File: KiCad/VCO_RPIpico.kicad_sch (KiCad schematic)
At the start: 30 parts, among them J1 AudioJack2, J2 Power Jack 5V, J3 Wave Out, J4 Echo Out, J5 Poti Echo Mix/Feedback, J6 Poti Echo Freq, J7 Echo Power, SW1 LFO Waveform, SW2 Shift1, SW3 Fire4, SW4 Fire3, SW5 Fire2, SW6 Fire1, SW7 Shift2, SW8 Shift3

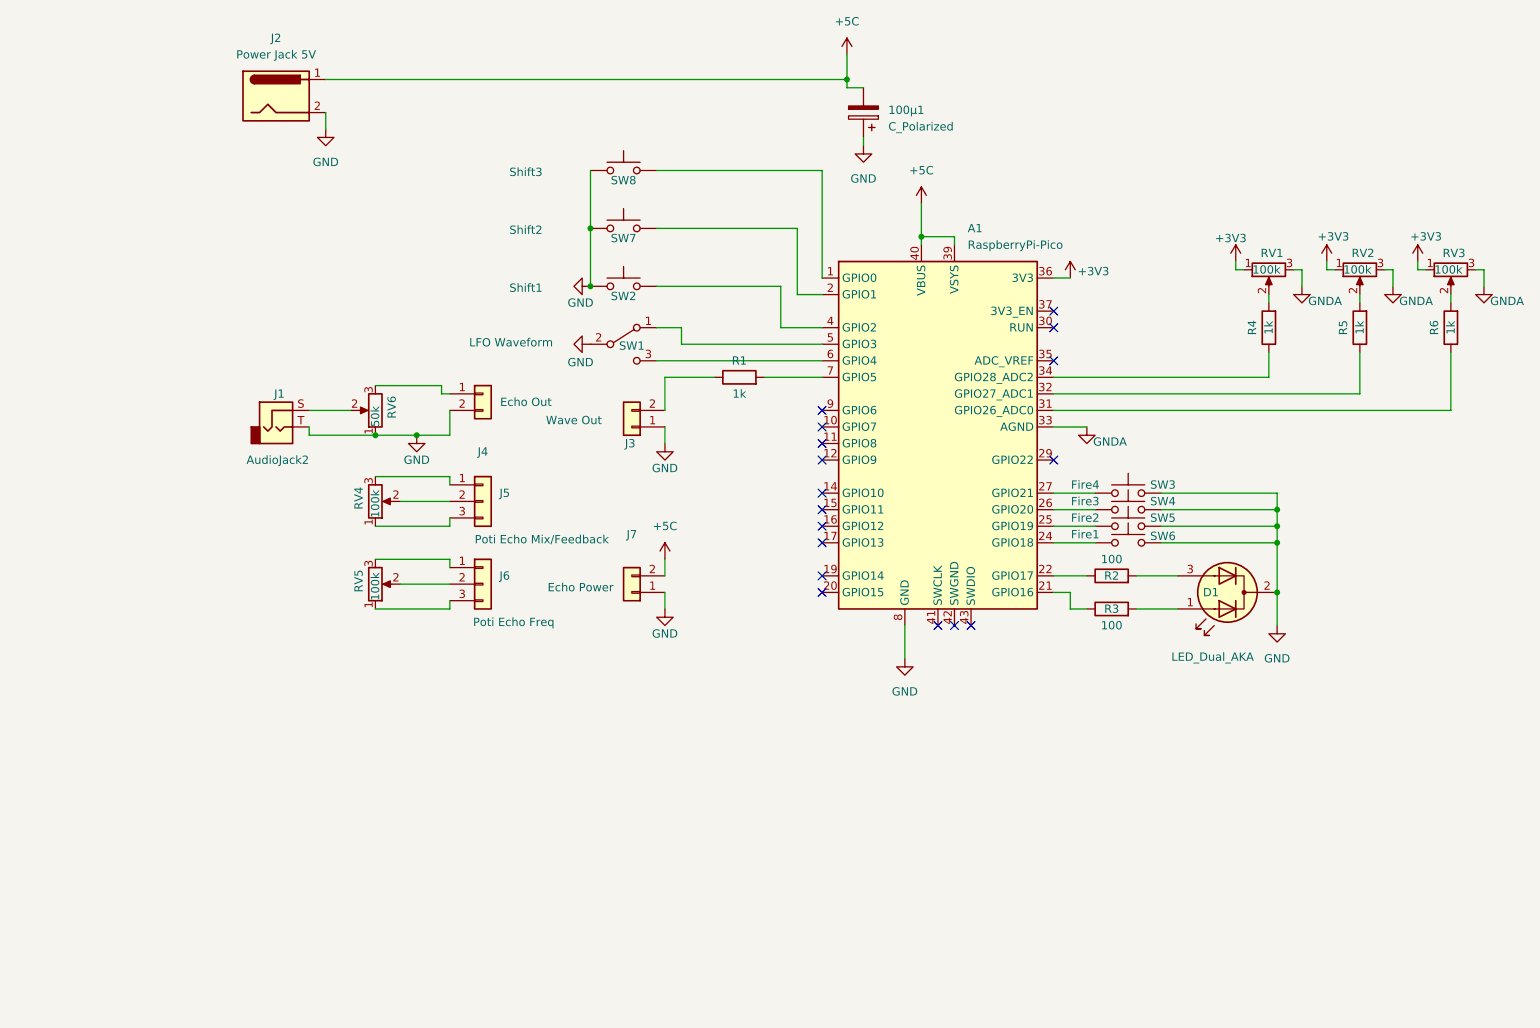
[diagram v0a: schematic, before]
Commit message: Kicad Schematic and Board
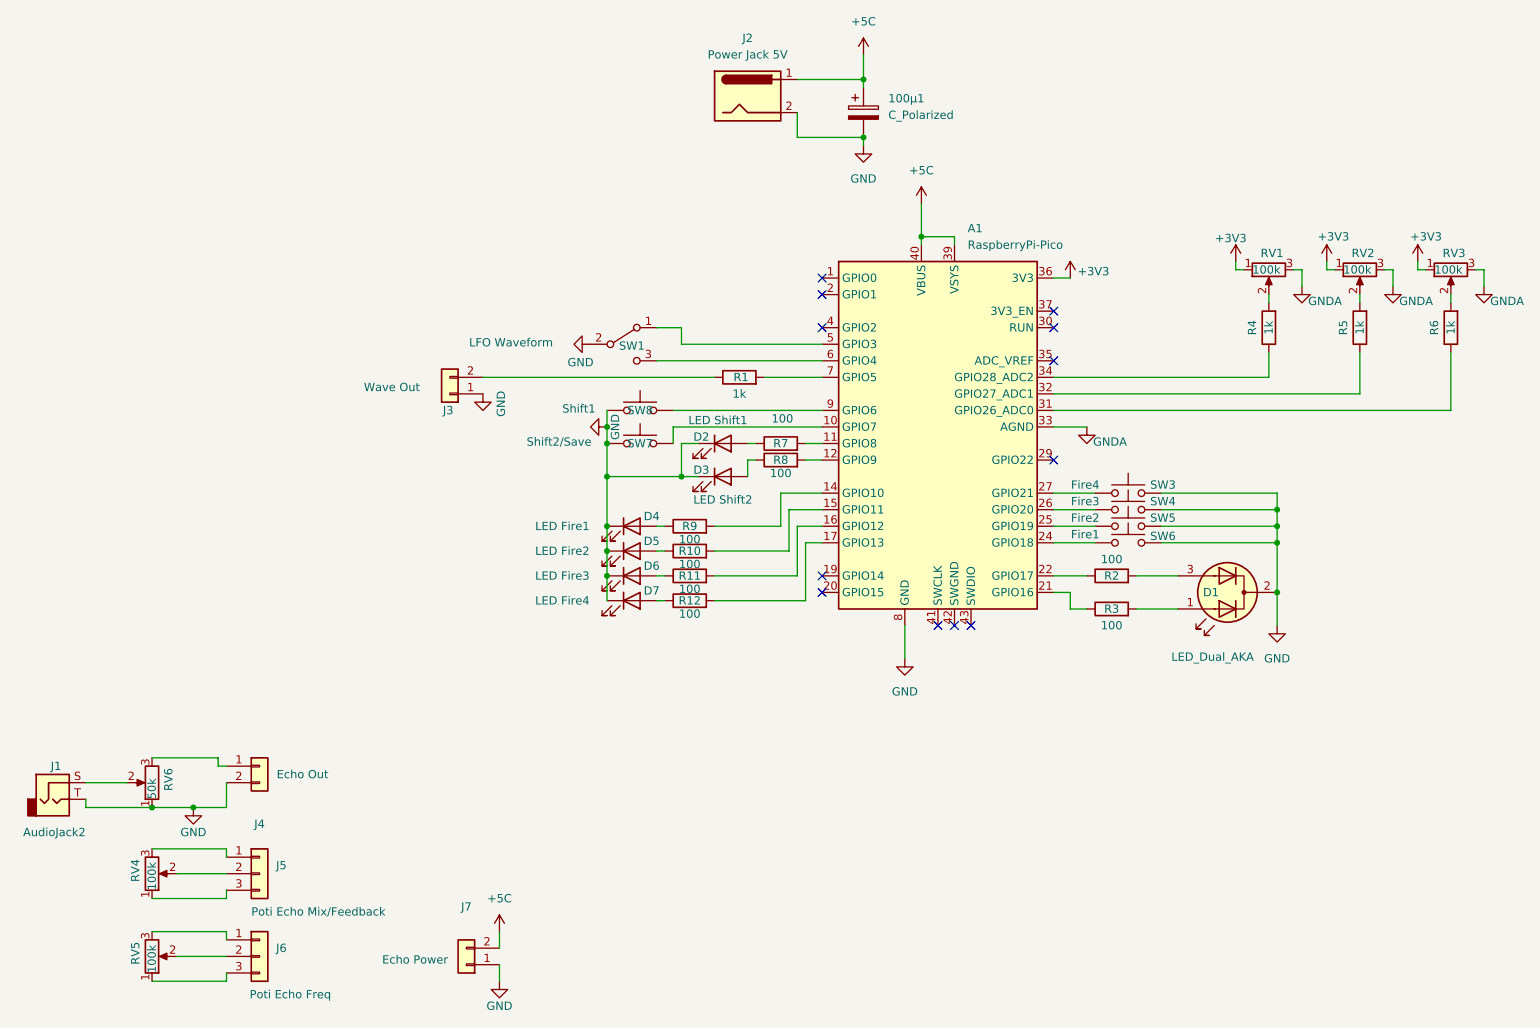
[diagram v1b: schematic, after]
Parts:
- removed SW2: Shift1, symbol Switch:SW_Push
- added D2: LED Shift1, LED_THT:LED_D3.0mm, symbol Device:LED
- added D3: LED Shift2, LED_THT:LED_D3.0mm, symbol Device:LED
- added D4: LED Fire1, LED_THT:LED_D3.0mm, symbol Device:LED
- added D5: LED Fire2, LED_THT:LED_D3.0mm, symbol Device:LED
- added D6: LED Fire3, LED_THT:LED_D3.0mm, symbol Device:LED
- added D7: LED Fire4, LED_THT:LED_D3.0mm, symbol Device:LED
- added R10, R11, R12, R7, R8, R9: 100, Resistor_SMD:R_1206_3216Metric, symbol Device:R
- A1: footprint RPI:Raspberry_Pi_Pico_THT -> RPI:Raspberry_Pi_Pico_SMT_THT
- J3, J4, J7: footprint (none) -> Connector_PinSocket_2.54mm:PinSocket_1x02_P2.54mm_Vertical
- J5, J6: footprint (none) -> Connector_PinSocket_2.54mm:PinSocket_1x03_P2.54mm_Vertical
- R1, R2, R3, R4, R5, R6: footprint Resistor_SMD:R_0603_1608Metric -> Resistor_SMD:R_1206_3216Metric
- SW1: footprint (none) -> Button_Switch_THT:SW_Slide-03_Wuerth-WS-SLTV_10x2.5x6.4_P2.54mm
- SW3, SW4, SW5, SW6: footprint (none) -> Button_Switch_THT:SW_PUSH_6mm
- SW7: value Shift2 -> Shift2/Save; footprint (none) -> Button_Switch_THT:SW_PUSH_6mm
- SW8: value Shift3 -> Shift1; footprint (none) -> Button_Switch_THT:SW_PUSH_6mm
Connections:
- net +5C: now also 100µ1.1; no longer 100µ1.2
- net GND: now also 100µ1.2, D2.1 (K), D3.1 (K), D4.1 (K), D5.1 (K), D6.1 (K), D7.1 (K); no longer 100µ1.1
- net at A1.1 (GPIO0): no longer SW8.2
- net at A1.10 (GPIO7): now also SW7.2
- net at A1.11 (GPIO8): now also R7.2
- net at A1.12 (GPIO9): now also R8.2
- net at A1.14 (GPIO10): now also R9.2
- net at A1.15 (GPIO11): now also R10.2
- net at A1.16 (GPIO12): now also R11.2
- net at A1.17 (GPIO13): now also R12.2
- net at A1.2 (GPIO1): no longer SW7.2
- net at A1.9 (GPIO6): now also SW8.2
- new net: D6.2 (A), R11.1
- new net: D4.2 (A), R9.1
- new net: D5.2 (A), R10.1
- new net: D2.2 (A), R7.1
- new net: D7.2 (A), R12.1
- new net: D3.2 (A), R8.1
- no-connect marks 17 -> 12
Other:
- moved on the sheet: 100µ1, J1, J2, J3, J4, J5, J6, J7, RV4, RV5, RV6, SW7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
